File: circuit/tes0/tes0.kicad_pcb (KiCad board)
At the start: 2 copper layers, 34 parts, among them U1 SIM7000E, U2 FT232RL, U3 AMS1117-3.3

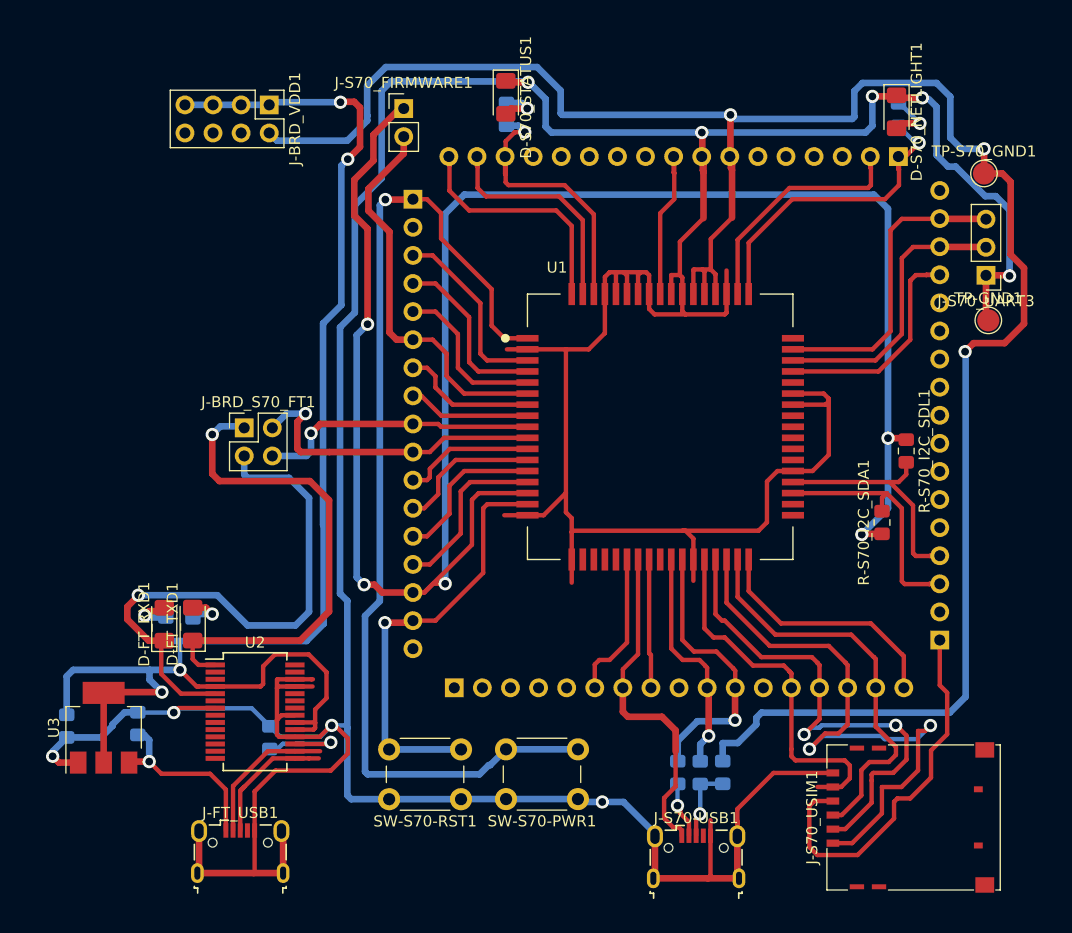
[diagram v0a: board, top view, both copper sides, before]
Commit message: update
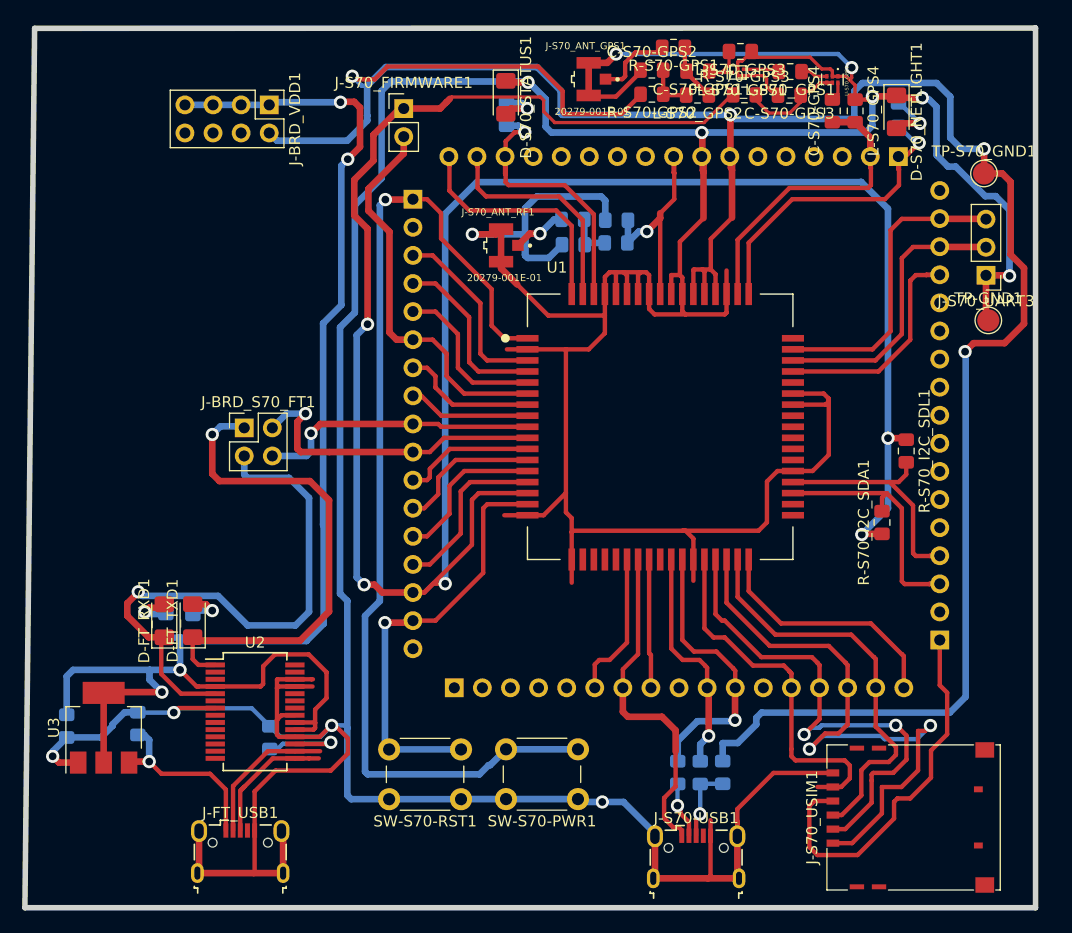
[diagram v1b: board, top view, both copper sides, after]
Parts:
- added C-S70-GPS1: 33pF, Capacitor_SMD:C_0805_2012Metric_Pad1.15x1.40mm_HandSolder, F.Cu at (189.8, 49.1)
- added C-S70-GPS2: 33pF, Capacitor_SMD:C_0805_2012Metric_Pad1.15x1.40mm_HandSolder, F.Cu at (185.7, 49.0)
- added C-S70-GPS3: 10pF, Capacitor_SMD:C_0805_2012Metric_Pad1.15x1.40mm_HandSolder, F.Cu at (198.1, 51.3)
- added C-S70-GPS4: 33pF, Capacitor_SMD:C_0805_2012Metric_Pad1.15x1.40mm_HandSolder, F.Cu at (202.0, 52.7)
- added C-S70_ANT_RF1: C, Capacitor_SMD:C_0805_2012Metric_Pad1.15x1.40mm_HandSolder, B.Cu at (178.6, 64.8)
- added C-S70_ANT_RF2: C, Capacitor_SMD:C_0805_2012Metric_Pad1.15x1.40mm_HandSolder, B.Cu at (182.5, 62.6)
- added FL-S70_GPS1: SAFFA1G58KA0F0A, Filter:Filter_1411-5_1.4x1.1mm, F.Cu at (193.4, 49.2)
- added J-S70_ANT_GPS1: 20279-001E-01, 20279-001E-01:IPEX_20279-001E-01, F.Cu at (180.0, 49.9)
- added J-S70_ANT_RF1: 20279-001E-01, 20279-001E-01:IPEX_20279-001E-01, F.Cu at (172.1, 64.9)
- added L-S70_ANT_RF1: L, Inductor_SMD:L_0805_2012Metric_Pad1.15x1.40mm_HandSolder, B.Cu at (182.4, 64.7)
- added L-S70_GPS1: L, Inductor_SMD:L_0805_2012Metric_Pad1.15x1.40mm_HandSolder, F.Cu at (198.2, 49.2)
- added L-S70_GPS2: L, Inductor_SMD:L_0805_2012Metric_Pad1.15x1.40mm_HandSolder, F.Cu at (189.8, 51.3)
- added L-S70_GPS3: L, Inductor_SMD:L_0805_2012Metric_Pad1.15x1.40mm_HandSolder, F.Cu at (193.7, 47.4)
- added L-S70_GPS4: L, Inductor_SMD:L_0805_2012Metric_Pad1.15x1.40mm_HandSolder, F.Cu at (204.1, 52.7)
- added R-S70-GPS1: 0, Resistor_SMD:R_0805_2012Metric_Pad1.15x1.40mm_HandSolder, F.Cu at (187.6, 47.0)
- added R-S70-GPS2: 10, Resistor_SMD:R_0805_2012Metric_Pad1.15x1.40mm_HandSolder, F.Cu at (185.7, 51.2)
- added R-S70-GPS3: 10, Resistor_SMD:R_0805_2012Metric_Pad1.15x1.40mm_HandSolder, F.Cu at (194.1, 51.3)
- added R-S70_ANT_RF1: 0, Resistor_SMD:R_0805_2012Metric_Pad1.15x1.40mm_HandSolder, B.Cu at (178.5, 62.5)
- added U-S70_GPS1: BGU7005,115, BGU7005_115:PSON50P145X100X50-6N, F.Cu at (202.0, 49.9)
- moved D-FT_TXD1 0.31 mm to (144.2, 98.8)
- moved R-FT_RXD1 0.31 mm to (144.2, 99.3)
- moved R-FT_TXD1 0.31 mm to (141.7, 99.2)
- moved D-FT_RXD1 0.31 mm to (141.6, 98.8)
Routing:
- net GND: track 439.2 -> 537.4 mm, vias 9 -> 12
- net /S70_VDDEXT: track 178.4 -> 212.6 mm
- net /S70_VDD: track 185.9 -> 218.0 mm, vias 3 -> 4
- net Net-(C-S70-GPS3-Pad1): track 0.00 -> 9.36 mm
- net Net-(J-S70_ANT_GPS1-Pad1): track 0.00 -> 7.03 mm
- net /S70_ANT_RF: track 13.9 -> 20.3 mm, vias 0 -> 1
- net /S70_ANT_GPS: track 22.1 -> 27.8 mm
- net Net-(C-S70-GPS1-Pad2): track 0.00 -> 5.23 mm
- net Net-(J-S70_ANT_RF1-Pad1): track 0.00 -> 4.92 mm, vias 0 -> 1
- net Net-(C-S70-GPS1-Pad1): track 0.00 -> 4.30 mm
- net Net-(C-S70-GPS2-Pad2): track 0.00 -> 4.29 mm
- net Net-(C-S70_ANT_RF1-Pad2): track 0.00 -> 4.18 mm
- net /S70_GPS_IN: track 0.00 -> 3.30 mm
- net Net-(L-S70_GPS1-Pad1): track 0.00 -> 2.47 mm
- net Net-(C-S70-GPS4-Pad2): track 0.00 -> 2.06 mm
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- added copper zone on B.Cu, net (none)
- added copper zone on F.Cu, net (none)
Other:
- board outline added: 91.4 x 79.5 mm
